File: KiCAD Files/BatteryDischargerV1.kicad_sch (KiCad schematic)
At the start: 25 parts

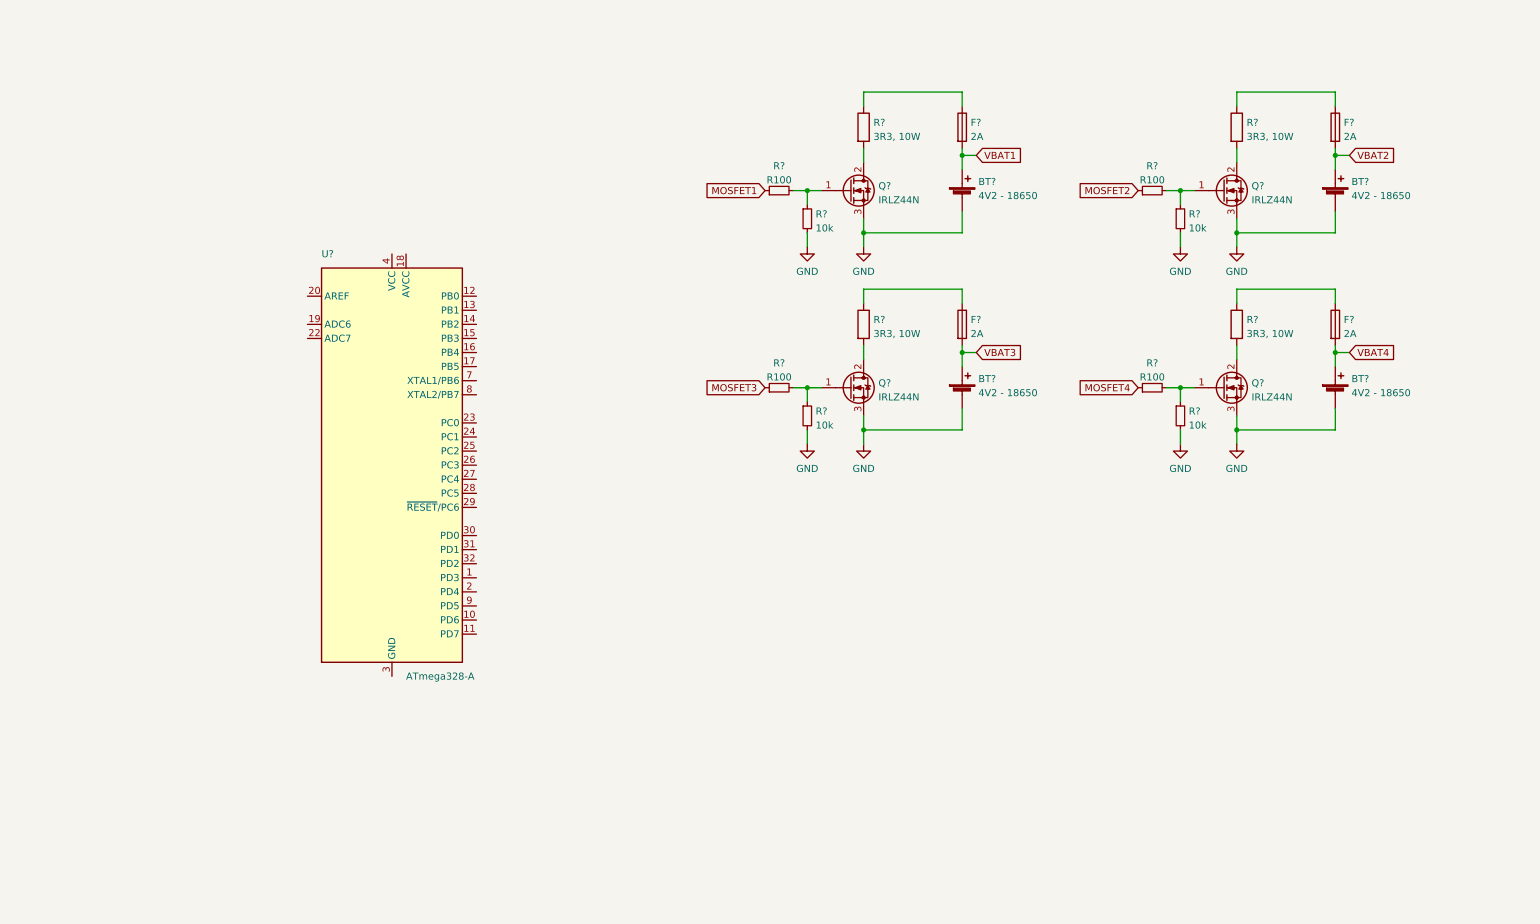
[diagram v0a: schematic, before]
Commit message: Update BatteryDischargerV1.kicad_sch
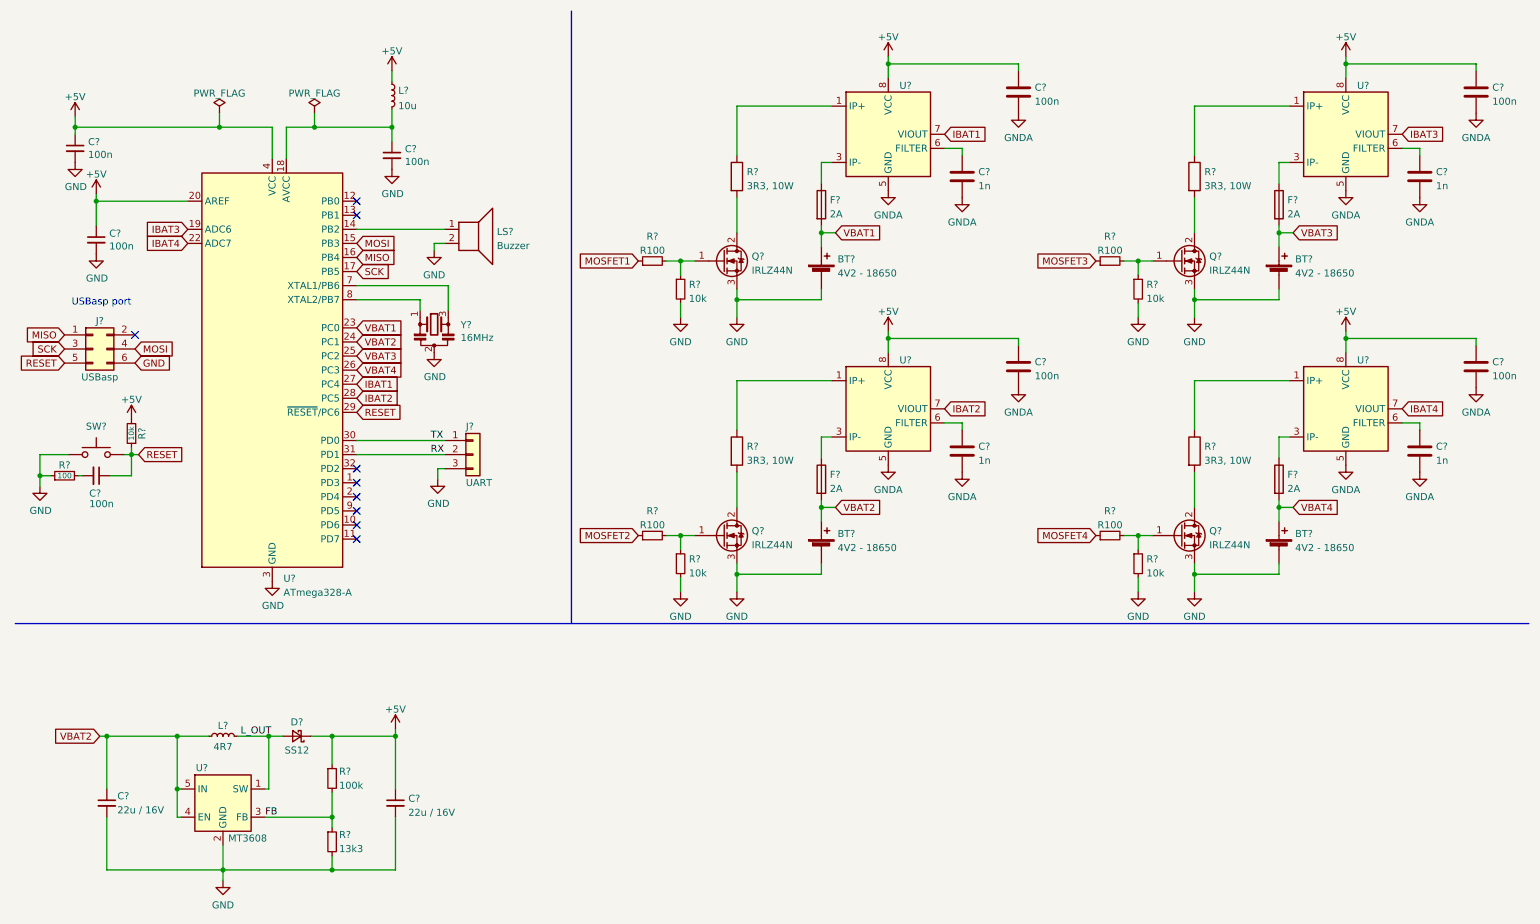
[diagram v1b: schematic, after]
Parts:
- removed BT? (x3): 4V2 - 18650, symbol Device:Battery_Cell
- removed F? (x3): 2A, symbol Device:Fuse
- removed Q? (x3): IRLZ44N, Package_TO_SOT_THT:TO-220-3_Vertical, symbol Transistor_FET:IRLZ44N
- removed R? (x3): 10k, symbol Device:R_Small
- removed R? (x3): R100, symbol Device:R_Small
- removed R? (x3): 3R3, 10W, symbol Device:R
- removed U?: ATmega328-A, Package_QFP:TQFP-32_7x7mm_P0.8mm, symbol MCU_Microchip_ATmega:ATmega328-A
- added BT? (x3): 4V2 - 18650, symbol Device:Battery_Cell
- added C? (x4): 100n, Capacitor_SMD:C_0805_2012Metric, symbol Device:C_Small
- added C? (x4): 100n, Capacitor_SMD:C_0603_1608Metric, symbol Device:C
- added C? (x4): 1n, Capacitor_SMD:C_0603_1608Metric, symbol Device:C
- added C? (x2): 22u / 16V, Capacitor_SMD:C_1210_3225Metric, symbol Device:C_Small
- added D?: SS12, Diode_SMD:D_SMA, symbol Device:D_Schottky_Small
- added F? (x3): 2A, symbol Device:Fuse
- added J?: UART, symbol Connector_Generic:Conn_01x03
- added J?: USBasp, Connector_PinSocket_1.27mm:PinSocket_2x03_P1.27mm_Vertical, symbol Connector_Generic:Conn_02x03_Odd_Even
- added L?: 4R7, Footprints:Inductor_4mm(5x5mm pads), symbol Device:L_Small
- added L?: 10u, Inductor_SMD:L_1206_3216Metric, symbol Device:L_Small
- added LS?: Buzzer, CNLJS:KLJ-1102, symbol Device:Speaker
- added Q? (x3): IRLZ44N, Package_TO_SOT_THT:TO-220-3_Vertical, symbol Transistor_FET:IRLZ44N
- added R? (x3): 3R3, 10W, symbol Device:R
- added R?: 100k, Resistor_SMD:R_0603_1608Metric, symbol Device:R_Small
- added R? (x3): 10k, symbol Device:R_Small
- added R? (x3): R100, symbol Device:R_Small
- added R?: 10k, Resistor_SMD:R_0603_1608Metric, symbol Device:R_Small
- added R?: 100, Resistor_SMD:R_0603_1608Metric, symbol Device:R_Small
- added R?: 13k3, Resistor_SMD:R_0603_1608Metric, symbol Device:R_Small
- added SW?: SW_Push, Button_Switch_SMD:SW_SPST_TL3342, symbol Switch:SW_Push
- added U? (x4): ACS712xLCTR-05B, Package_SO:SOIC-8_3.9x4.9mm_P1.27mm, symbol Sensor_Current:ACS712xLCTR-05B
- added U?: ATmega328-A, Package_QFP:TQFP-32_7x7mm_P0.8mm, symbol MCU_Microchip_ATmega:ATmega328-A
- added U?: MT3608, Package_TO_SOT_SMD:SOT-23-6, symbol Regulator_Switching:MT3608
- added Y?: 16MHz, CNLJS:CSTCE16M0V53-R0, symbol Device:Resonator_Small
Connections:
- net GND: now also BT?.2 (-), BT?.2 (-), BT?.2 (-), C?.2, C?.2, C?.2, C?.2, C?.2, J?.3 (Pin_3), J?.6 (Pin_6), LS?.2, Q?.3 (S), Q?.3 (S), Q?.3 (S), R?.1, R?.2, R?.2, R?.2, R?.2, SW?.1, U?.2 (GND), U?.21 (GND), U?.3 (GND), U?.5 (GND), Y?.2
- net MOSFET2: now also R?.1
- net MOSFET3: now also R?.1
- net MOSFET4: now also R?.1
- net VBAT1: now also U?.23 (PC0)
- net VBAT2: now also BT?.1 (+), C?.1, F?.2, L?.1, U?.24 (PC1), U?.4 (EN), U?.5 (IN)
- net VBAT3: now also BT?.1 (+), F?.2, U?.25 (PC2)
- net VBAT4: now also BT?.1 (+), F?.2, U?.26 (PC3)
- net at F?.1: now also U?.3 (IP-), U?.4 (IP-); no longer R?.1
- new net: R?.1, U?.1 (IP+), U?.2 (IP+) (x4)
- new net: Q?.2 (D), R?.2 (x3)
- new net: C?.2, R?.2
- new net: Q?.1 (G), R?.1, R?.2 (x3)
- new net: F?.1, U?.3 (IP-), U?.4 (IP-) (x3)
- new net: C?.1, U?.6 (FILTER) (x4)
- new net: U?.8 (XTAL2/PB7), Y?.1
- new net: U?.7 (XTAL1/PB6), Y?.3
- new net: LS?.1, U?.14 (PB2)
- new net: C?.1, L?.2, U?.18 (AVCC)
- new net +5V: C?.1, C?.1, C?.1, C?.1, C?.1, C?.1, C?.1, D?.1 (K), L?.1, R?.1, R?.2, U?.20 (AREF), U?.4 (VCC), U?.6 (VCC), U?.8 (VCC), U?.8 (VCC), U?.8 (VCC), U?.8 (VCC)
- new net FB: R?.1, R?.2, U?.3 (FB)
- new net GNDA: C?.2, C?.2, C?.2, C?.2, C?.2, C?.2, C?.2, C?.2, U?.5 (GND), U?.5 (GND), U?.5 (GND), U?.5 (GND)
- new net IBAT1: U?.27 (PC4), U?.7 (VIOUT)
- new net IBAT2: U?.28 (PC5), U?.7 (VIOUT)
- new net IBAT3: U?.19 (ADC6), U?.7 (VIOUT)
- new net IBAT4: U?.22 (ADC7), U?.7 (VIOUT)
- new net L_OUT: D?.2 (A), L?.2, U?.1 (SW)
- new net MISO: J?.1 (Pin_1), U?.16 (PB4)
- new net MOSI: J?.4 (Pin_4), U?.15 (PB3)
- new net RESET: C?.1, J?.5 (Pin_5), R?.1, SW?.2, U?.29 (~{RESET}/PC6)
- new net RX: J?.2 (Pin_2), U?.31 (PD1)
- new net SCK: J?.3 (Pin_3), U?.17 (PB5)
- new net TX: J?.1 (Pin_1), U?.30 (PD0)
- no-connect marks 0 -> 9
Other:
- note added: "USBasp port"
- moved on the sheet: BT?, F?, Q?, R?
